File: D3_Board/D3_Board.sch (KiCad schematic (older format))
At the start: 25 parts, among them J1 LED_Matrix, J2 MOTOR1, J3 MOTOR2, M1 Motor_Servo, M2 Motor_Servo, U1 LM2596_module, U2 ChinaBluePill, U3 LM2596_module

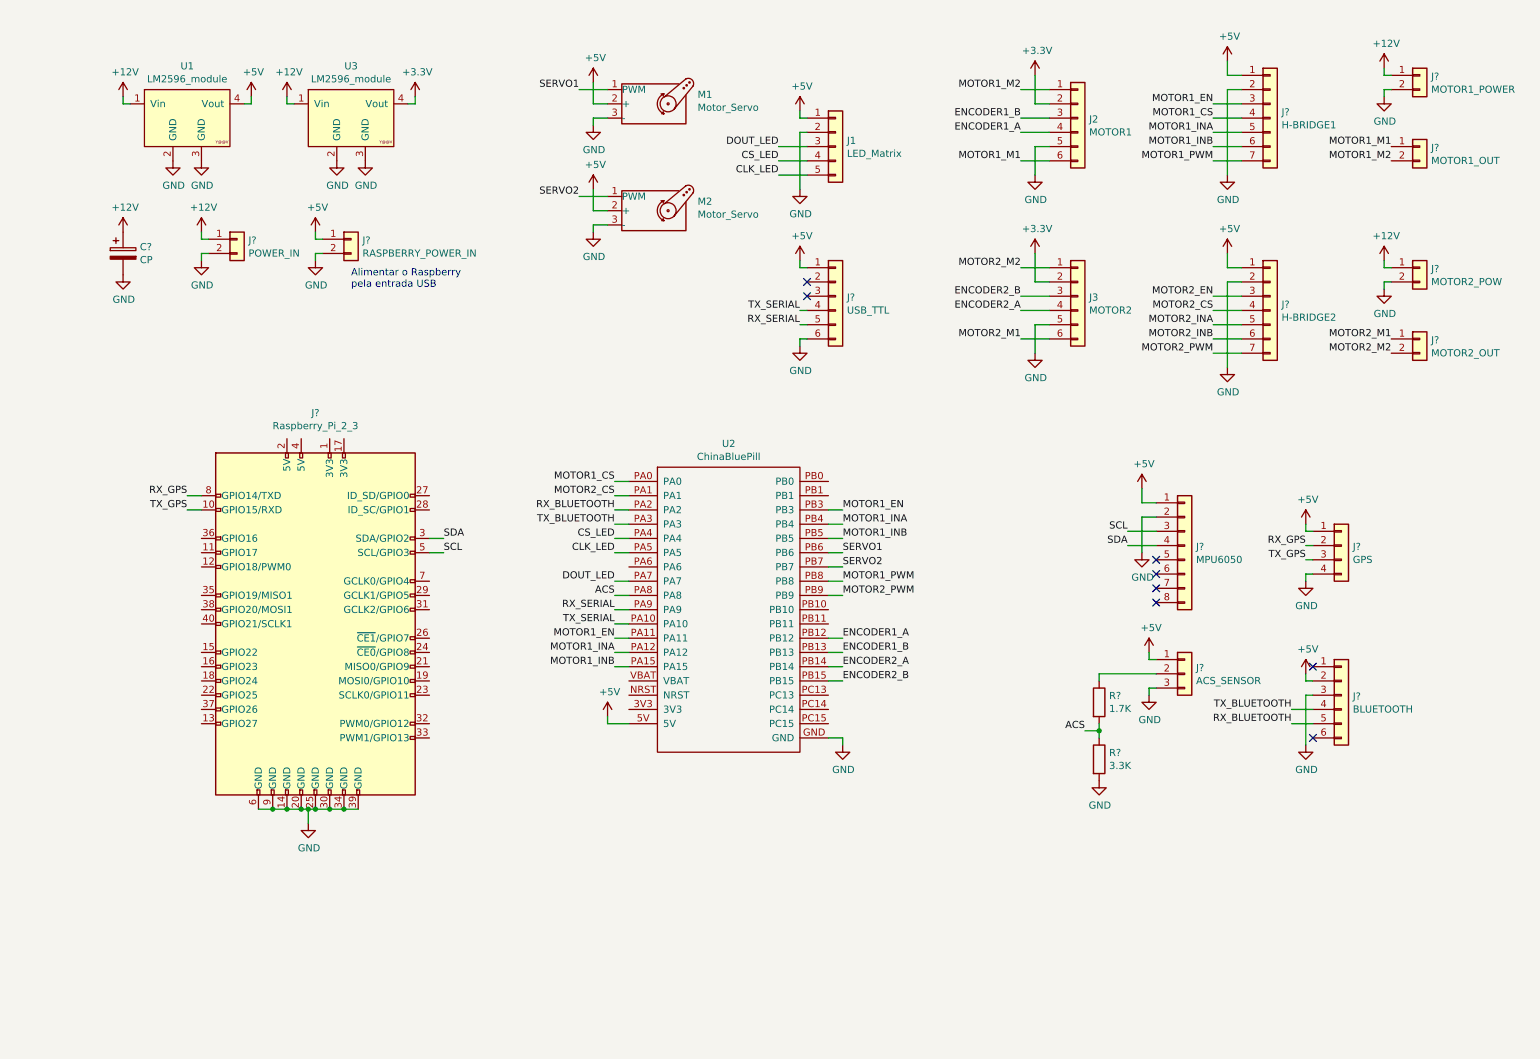
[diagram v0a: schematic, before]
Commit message: Finish schematics
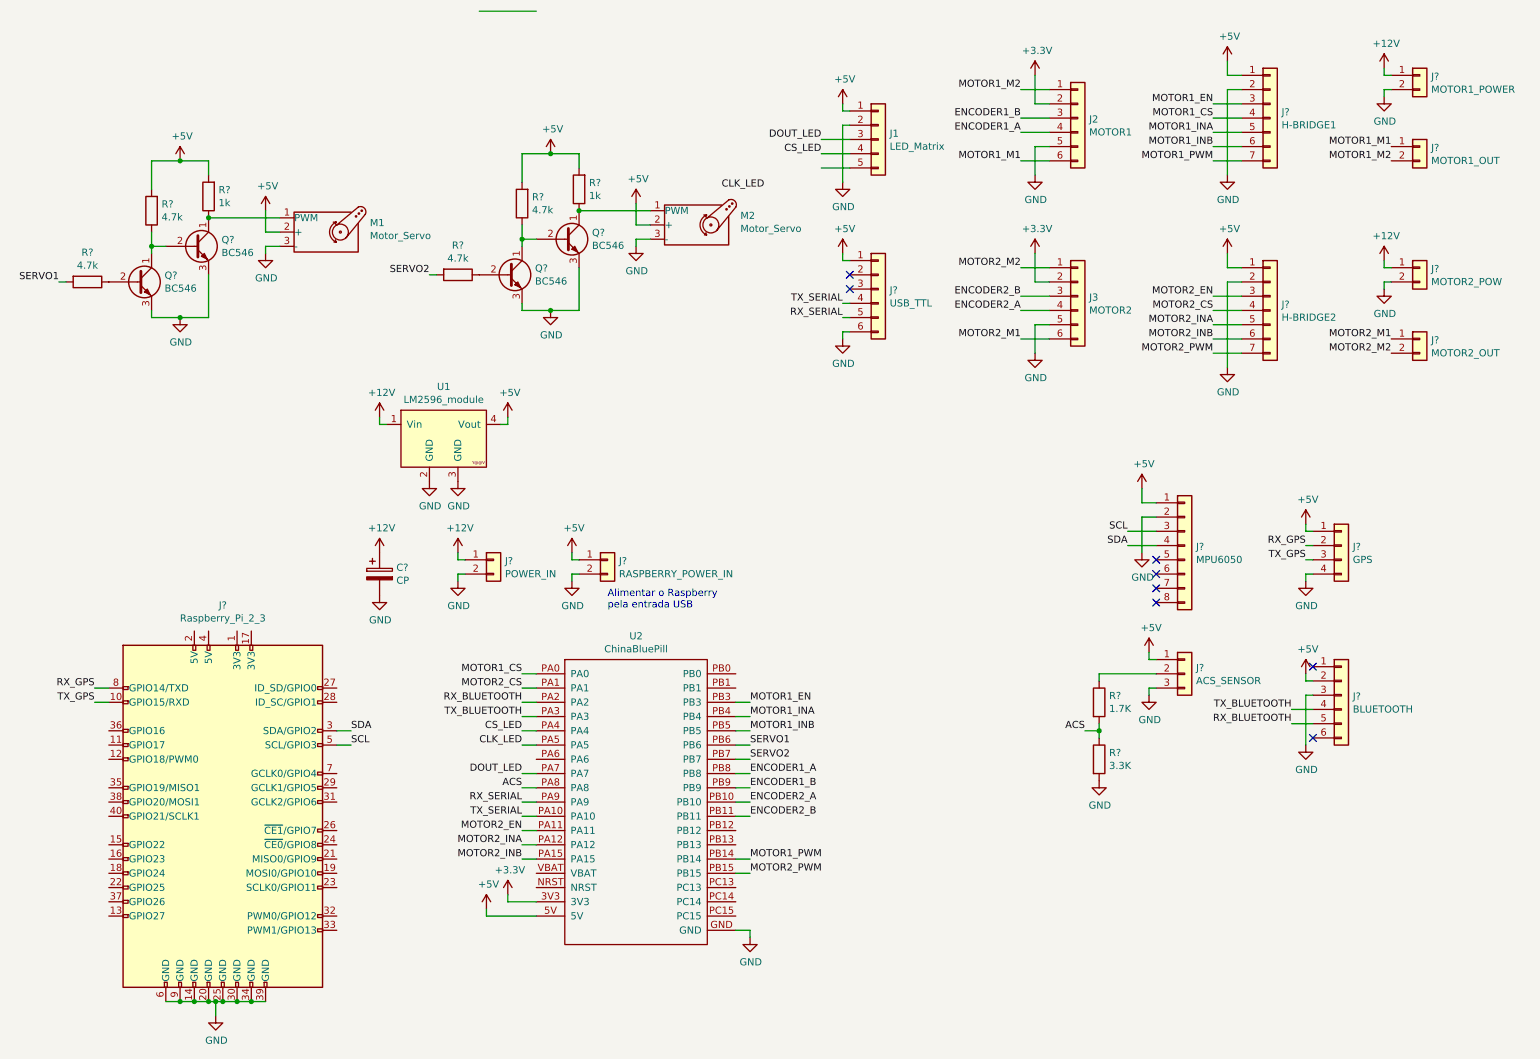
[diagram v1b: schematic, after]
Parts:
- removed U3: LM2596_module, LM2596:lm2596_module, symbol D3_Board:YAAJ_DCDC_StepUp_SX1308-lm2596_module
- added Q? (x4): BC546, Package_TO_SOT_THT:TO-92_Inline, symbol Transistor_BJT:BC546
- added R? (x4): 4.7k, symbol Device:R
- added R? (x2): 1k, symbol Device:R
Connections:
- net +3V3: now also U2.3V3
- net +5V: now also R?.2, R?.2, R?.2, R?.2
- net CLK_LED: no longer J1.5 (Pin_5)
- net ENCODER1_A: now also U2.PB8; no longer U2.PB12
- net ENCODER1_B: now also U2.PB9; no longer U2.PB13
- net ENCODER2_A: now also U2.PB10; no longer U2.PB14
- net ENCODER2_B: now also U2.PB11; no longer U2.PB15
- net GND: now also Q?.3 (E), Q?.3 (E), Q?.3 (E), Q?.3 (E)
- net MOTOR1_EN: no longer U2.PA11
- net MOTOR1_INA: no longer U2.PA12
- net MOTOR1_INB: no longer U2.PA15
- net MOTOR1_PWM: now also U2.PB14; no longer U2.PB8
- net MOTOR2_EN: now also U2.PA11
- net MOTOR2_INA: now also U2.PA12
- net MOTOR2_INB: now also U2.PA15
- net MOTOR2_PWM: now also U2.PB15; no longer U2.PB9
- net SERVO1: now also R?.2; no longer M1.1 (PWM)
- net SERVO2: now also R?.2; no longer M2.1 (PWM)
- new net: M1.1 (PWM), Q?.1 (C), R?.1
- new net: M2.1 (PWM), Q?.1 (C), R?.1
- new net: Q?.2 (B), R?.1 (x2)
- new net: Q?.1 (C), Q?.2 (B), R?.1 (x2)
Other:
- moved on the sheet: C?, J1, J?, M1, M2, U1, U2
